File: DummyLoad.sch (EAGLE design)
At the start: 16 parts, among them IC1 LM358, J1 BINDING-POST, J2 BINDING-POST, Q1 NTE2390-OFFBOARD, SW1 SWITCH-SPDT, X1 SCREW-TERM-2

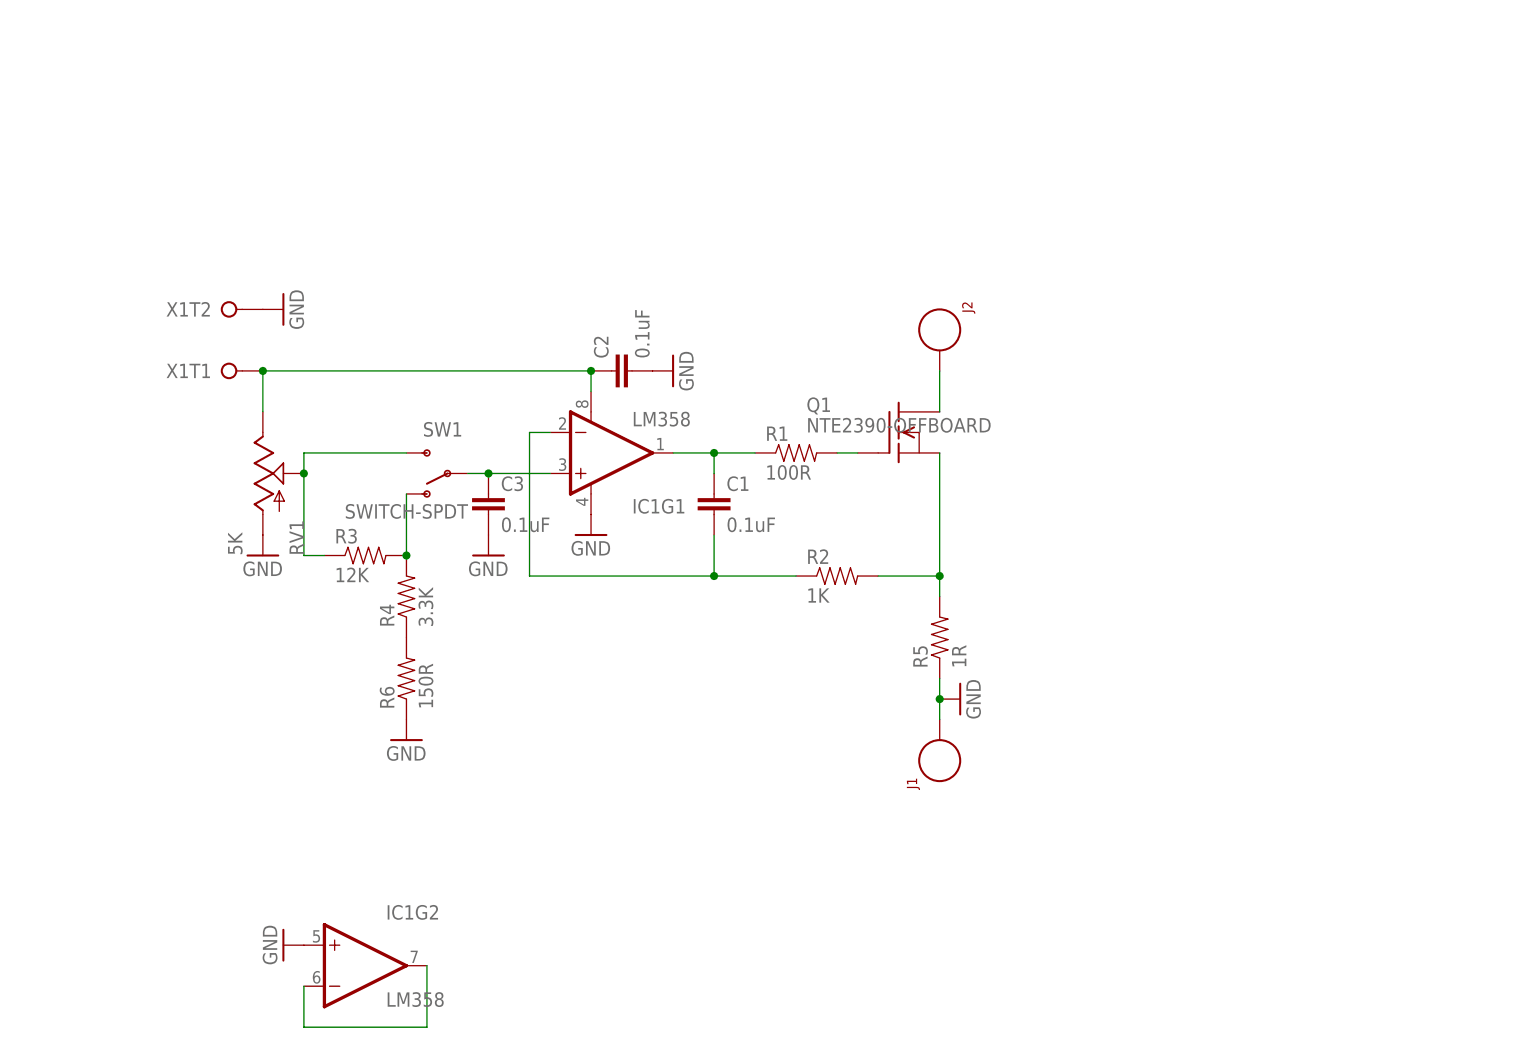
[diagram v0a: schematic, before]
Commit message: Rough layout
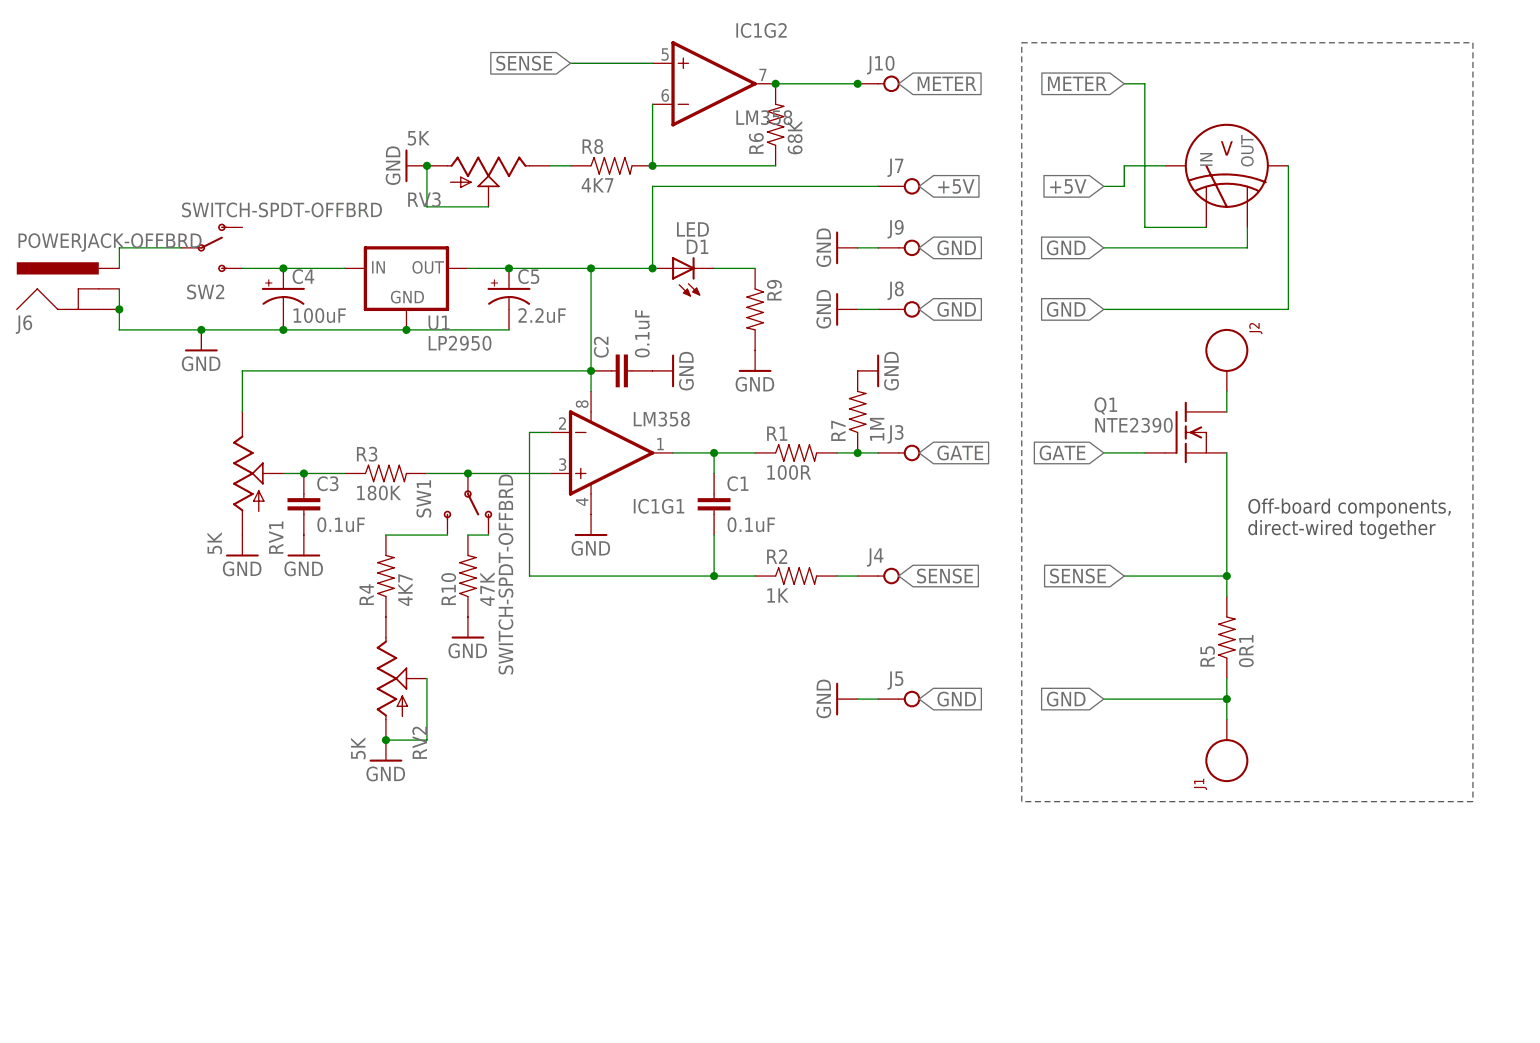
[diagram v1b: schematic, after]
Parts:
- removed X1: SCREW-TERM-2, SaintGimp:SCREW-TERM-2
- added C4: 100uF, SaintGimp:CAP-POL-5-8
- added C5: 2.2uF, SaintGimp:CAP-POL-2.5-5
- added D1: LED, SaintGimp:LED
- added J10, J3, J4, J5, J7, J8, J9: PINHD-1X1, SaintGimp:PINHD-1X1
- added J6: POWERJACK-OFFBRD, SaintGimp:POWERJACK-OFFBRD
- added R10: 47K, SaintGimp:RESISTOR-7.5MM
- added R7: 1M, SaintGimp:RESISTOR-7.5MM
- added R8: 4K7, SaintGimp:RESISTOR-7.5MM
- added R9: (no value), SaintGimp:RESISTOR-7.5MM
- added RV2, RV3: 5K, SaintGimp:POTTRIM
- added SW2: SWITCH-SPDT-OFFBRD, SaintGimp:SWITCH-SPDT-OFFBRD
- added U$1: PANEL-METER-OFFBRD, SaintGimp:PANEL-METER-OFFBRD
- added U1: LP2950, SaintGimp:LP2950
- Q1: value NTE2390-OFFBOARD -> NTE2390; device SaintGimp:NTE2390-OFFBOARD -> SaintGimp:NTE2390
- R3: value 12K -> 180K
- R4: value 3.3K -> 4K7
- R5: value 1R -> 0R1; device SaintGimp:RESISTOR-OFFBOARD -> SaintGimp:RESISTOR-7.5MM
- R6: value 150R -> 68K
- RV1: device SaintGimp:POT-PCB-MOUNT -> SaintGimp:POT-OFFBRD
- SW1: value SWITCH-SPDT -> SWITCH-SPDT-OFFBRD; device SaintGimp:SWITCH-SPDT -> SaintGimp:SWITCH-SPDT-OFFBRD
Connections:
- removed net N$2 (its old number): Q1.GATE, R1.2
- new net +5V: C2.1, C5.+, D1.A, IC1G1.V+, J7.KL, RV1.E, U$1.5V, U1.OUT
- new net GATE: J3.KL, Q1.GATE, R1.2, R7.1
- new net METER: IC1G2.OUT, J10.KL, R6.2, U$1.IN
- new net N$12: R8.1, RV3.E
- new net N$13: IC1G1.+IN, R3.2, SW1.P
- new net N$4: D1.C, R9.1
- new net SENSE: IC1G2.+IN, J4.KL, Q1.SRC, R2.2, R5.2
- net GND: now also C4.-, C5.-, J5.KL, J6.GND, J6.GNDBREAK, J8.KL, J9.KL, R10.1, R7.2, R9.2, RV2.A, RV2.S, RV3.A, RV3.S, U$1.GND, U$1.OUT, U1.GND; no longer IC1G2.+IN, R6.1, X1T2.KL
- net N$1: now also J6.PWR, SW2.P; no longer IC1G2.-IN, IC1G2.OUT
- net N$10: now also R4.2; no longer R3.1, RV1.S
- net N$11: now also RV2.E; no longer R6.2
- net N$3: now also C4.+, SW2.S, U1.IN; no longer Q1.SRC, R2.2, R5.2
- net N$6: now also C3.1, R3.1, RV1.S; no longer R3.2, R4.2, SW1.O
- net N$8: now also IC1G2.-IN, R6.1, R8.2; no longer C2.1, IC1G1.V+, RV1.E, X1T1.KL
- net N$9: now also R10.2, SW1.O; no longer C3.1, IC1G1.+IN, SW1.P
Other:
- note added: "Off-board components, direct-wired together"
- moved on the sheet: C3, IC1G2, J1, J2, Q1, R2, R3, R4, R5, R6, RV1, SW1
